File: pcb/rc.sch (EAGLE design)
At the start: 79 parts, among them IC2 TP4056

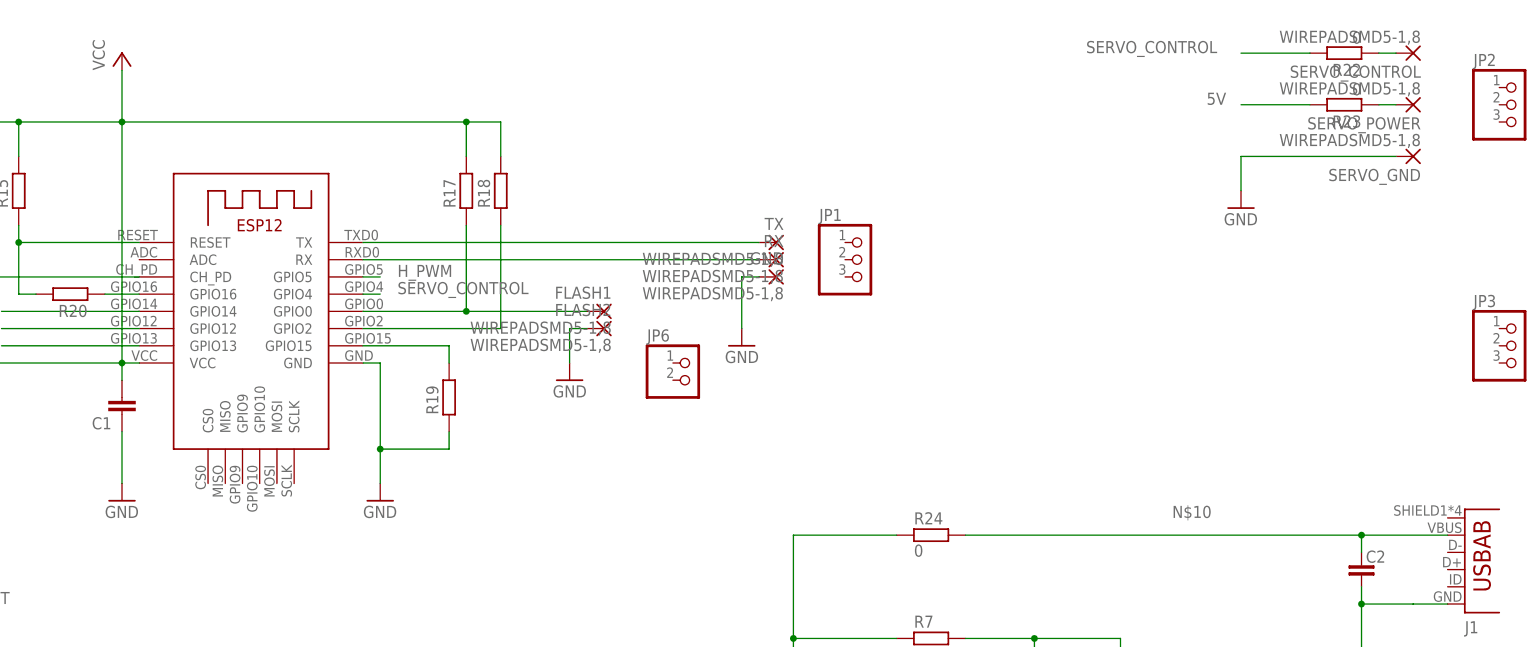
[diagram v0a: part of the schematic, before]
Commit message: pcb
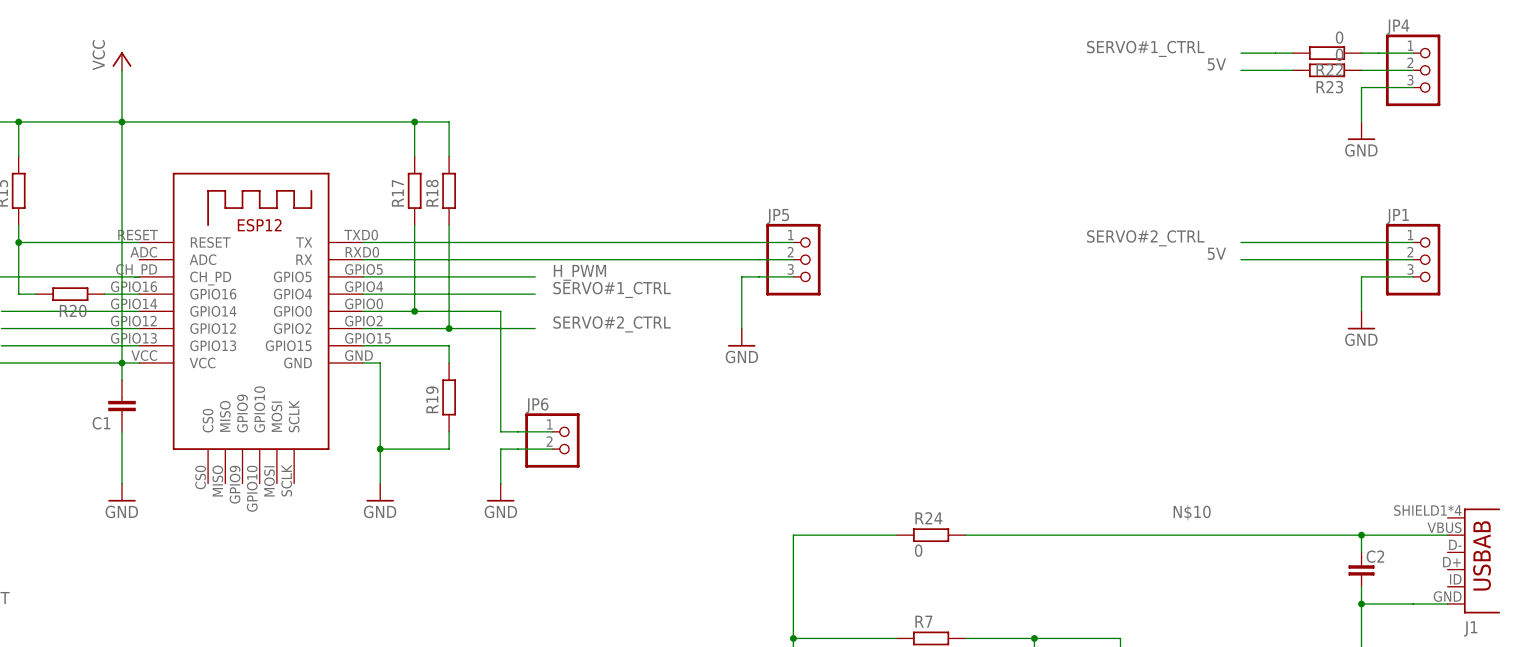
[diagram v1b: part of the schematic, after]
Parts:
- removed FLASH1, FLASH2, GND, RX, SERVO_CONTROL, SERVO_GND, SERVO_POWER, TX: WIREPADSMD5-1,8, wirepad:WIREPADSMD5-1,8
- removed JP2, JP3: (no value), pinhead:PINHD-1X3
- added JP4, JP5: (no value), my:PINHD-1X3
- JP1: device pinhead:PINHD-1X3 -> my:PINHD-1X3
- JP6: device pinhead:PINHD-1X2 -> my:PINHD-1X2
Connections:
- net SERVO_CONTROL renamed SERVO#1_CTRL
- removed net N$29: R22.1, SERVO_CONTROL.P
- new net SERVO#2_CTRL: JP1.1, R18.1, U1.GPIO2
- net 5V: now also JP1.2
- net GND: now also JP1.3, JP4.3, JP5.3, JP6.2; no longer FLASH2.P, GND.P, SERVO_GND.P
- net N$21: now also JP6.1; no longer FLASH1.P
- net N$22: now also JP4.1, R22.1; no longer R18.1, U1.GPIO2
- net N$30: now also JP4.2; no longer SERVO_POWER.P
- net RX: now also JP5.2; no longer RX.P
- net TX: now also JP5.1; no longer TX.P
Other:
- moved on the sheet: JP1, JP6, R17, R18, R22, R23
